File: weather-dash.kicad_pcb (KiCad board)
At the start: 11 copper layers, 61 x 45.5 mm, 13 parts, among them J1 Conn_01x02_Pin, J3 Conn_01x03_Socket, SW1 SW_Push, SW2 SW_SPDT, SW3 SW_Push, U1 WEMOS_C3_Mini, U2 TFT_ST7735_SD

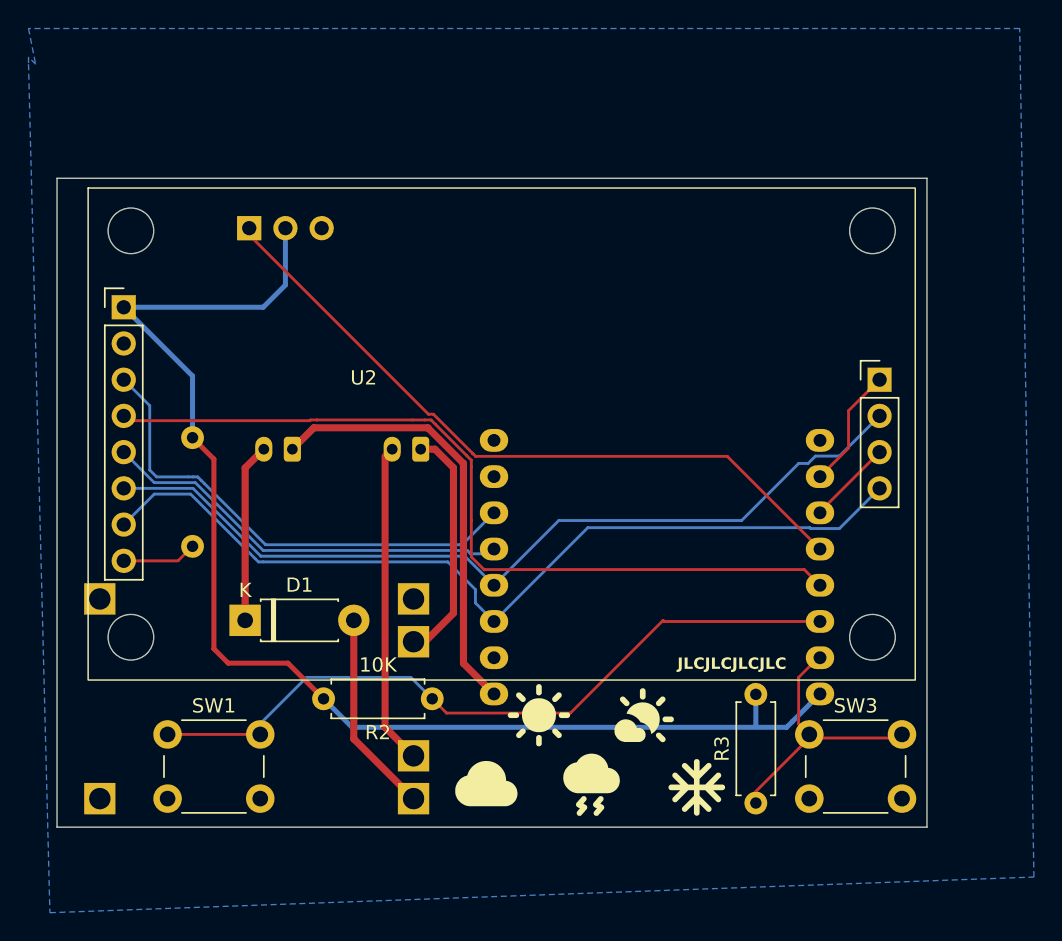
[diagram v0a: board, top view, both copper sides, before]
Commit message: more pcb changes
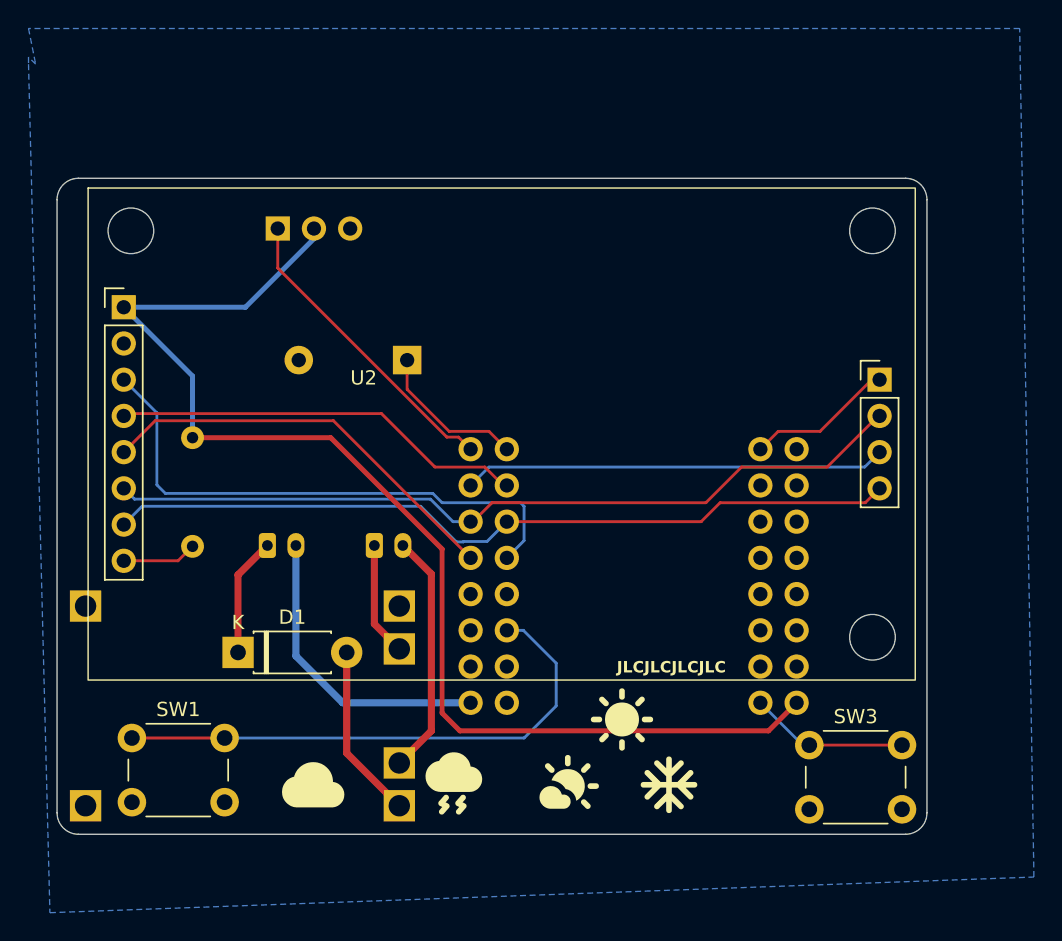
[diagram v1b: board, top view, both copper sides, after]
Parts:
- removed R2, R3: 10K, Resistor_THT:R_Axial_DIN0207_L6.3mm_D2.5mm_P7.62mm_Horizontal
- added BZ1: Buzzer, Buzzer_Beeper:Buzzer_12x9.5RM7.6, B.Cu at (39.5, 36.2)
- SW2: value SW_SPDT -> SW_SPST
- U1: value WEMOS_C3_Mini -> WEMOS_S2_Mini; footprint asylum-weather:WEMOS_C3_mini -> asylum-weather:WEMOS_S2_Mini
- moved J1 7.49 mm to (37.2, 49.2), turned to 0 degrees
- moved SW2 6.97 mm to (29.8, 49.2), turned to 0 degrees
- moved SW1 2.51 mm to (20.2, 62.8)
- moved D1 2.30 mm to (27.7, 56.8)
- moved J3 2.00 mm to (30.5, 27.0)
- moved G*** 2.00 mm to (67.0, 30.5)
- moved U1 1.75 mm to (55.4, 50.0)
- moved U3 1.12 mm to (28.5, 60.5)
- moved SW3 0.75 mm to (67.8, 63.2)
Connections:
- SW2 pad 1: VBUS -> Net-(D1-K)
- SW2 pad 2: Net-(D1-K) -> VBUS
- U1 pad 10: GND -> unconnected-(U1-IO2-Pad10)
- U1 pad 11: SCK -> unconnected-(U1-IO4-Pad11)
- U1 pad 12: MOSI -> unconnected-(U1-IO6-Pad12)
- U1 pad 13: TFT_DC -> unconnected-(U1-IO8-Pad13)
- U1 pad 14: TFT_CS -> unconnected-(U1-IO10/CS0-Pad14)
- U1 pad 16: unconnected-(U1-TX-Pad16) -> BTN2
- U1 pad 2: SD_CS -> unconnected-(U1-IO3-Pad2)
- U1 pad 3: MISO -> unconnected-(U1-IO5-Pad3)
- U1 pad 4: DHT11 -> unconnected-(U1-IO7-Pad4)
- U1 pad 5: TFT_EN -> unconnected-(U1-IO9-Pad5)
- U1 pad 6: BTN1 -> unconnected-(U1-IO11/MOSI-Pad6)
- U1 pad 7: BTN2 -> unconnected-(U1-IO12/SCK-Pad7)
- U1 pad 9: VBUS -> SD_CS
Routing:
- net TFT_EN: track 57.8 -> 29.0 mm
- net DHT11: track 49.9 -> 21.6 mm
- net MISO: track 5.99 -> 29.6 mm
- net BTN1: track 51.6 -> 38.1 mm
- net BUZ: track 0.00 -> 10.8 mm
- net VBUS: track 30.7 -> 21.4 mm
- net BAT-: track 16.7 -> 7.97 mm
- net BTN2: track 19.0 -> 11.5 mm
- net SCK: track 62.1 -> 56.1 mm
- net BAT+: track 22.5 -> 17.0 mm
- net +3.3V: track 90.4 -> 85.6 mm
- net TFT_CS: track 34.3 -> 38.8 mm
- net MOSI: track 60.7 -> 57.0 mm
- net Net-(D1-K): track 12.5 -> 9.10 mm
- net SD_CS: track 8.53 -> 10.4 mm
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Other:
- board size 61 x 45.5 mm -> 61 x 46 mm
- board text added: "v0.4"
- board text removed: "v0.2"
